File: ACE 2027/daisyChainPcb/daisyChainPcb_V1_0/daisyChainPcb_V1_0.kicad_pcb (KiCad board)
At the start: 2 copper layers, 56.5 x 97 mm, 27 parts, among them J201 Pads, J202 XT30, J203 XT30, J204 Pads, J205 Pads, J206 RJ45, J207 RJ45, U101 AP7361C-33E-13

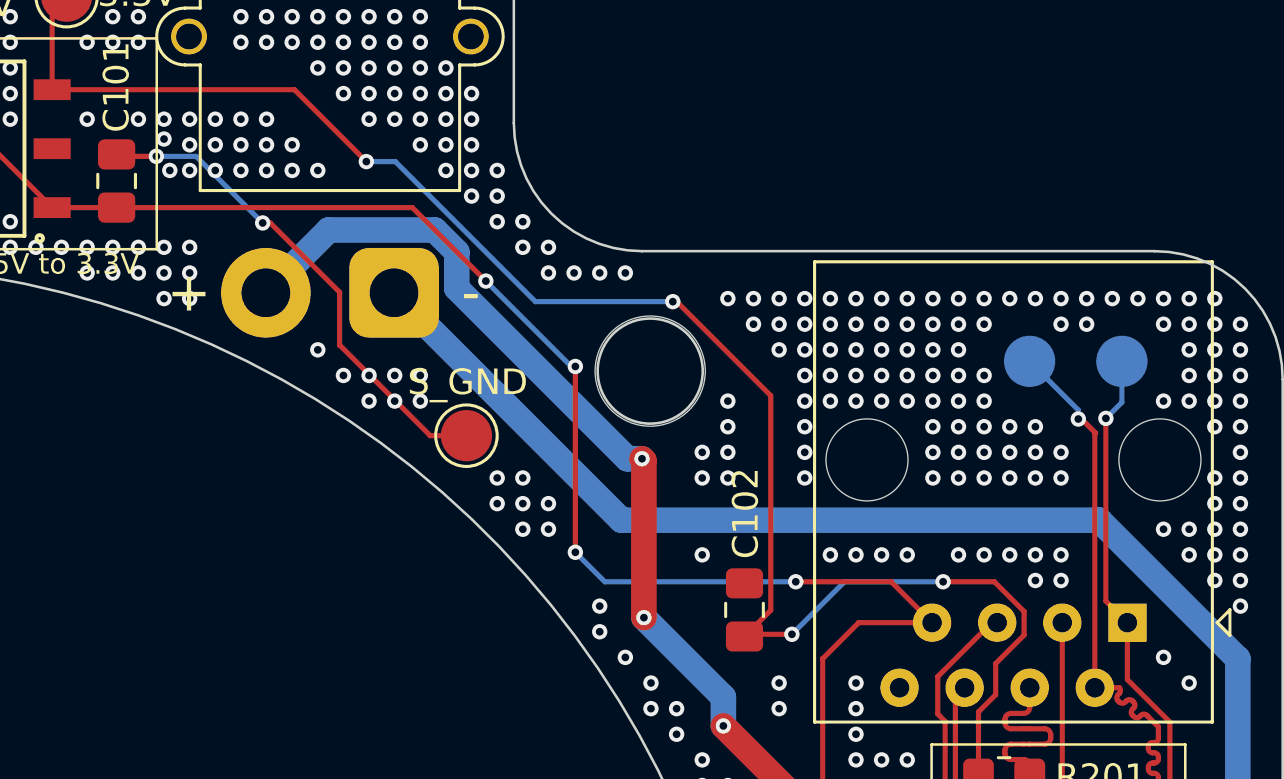
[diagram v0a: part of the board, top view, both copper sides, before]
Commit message: version finale
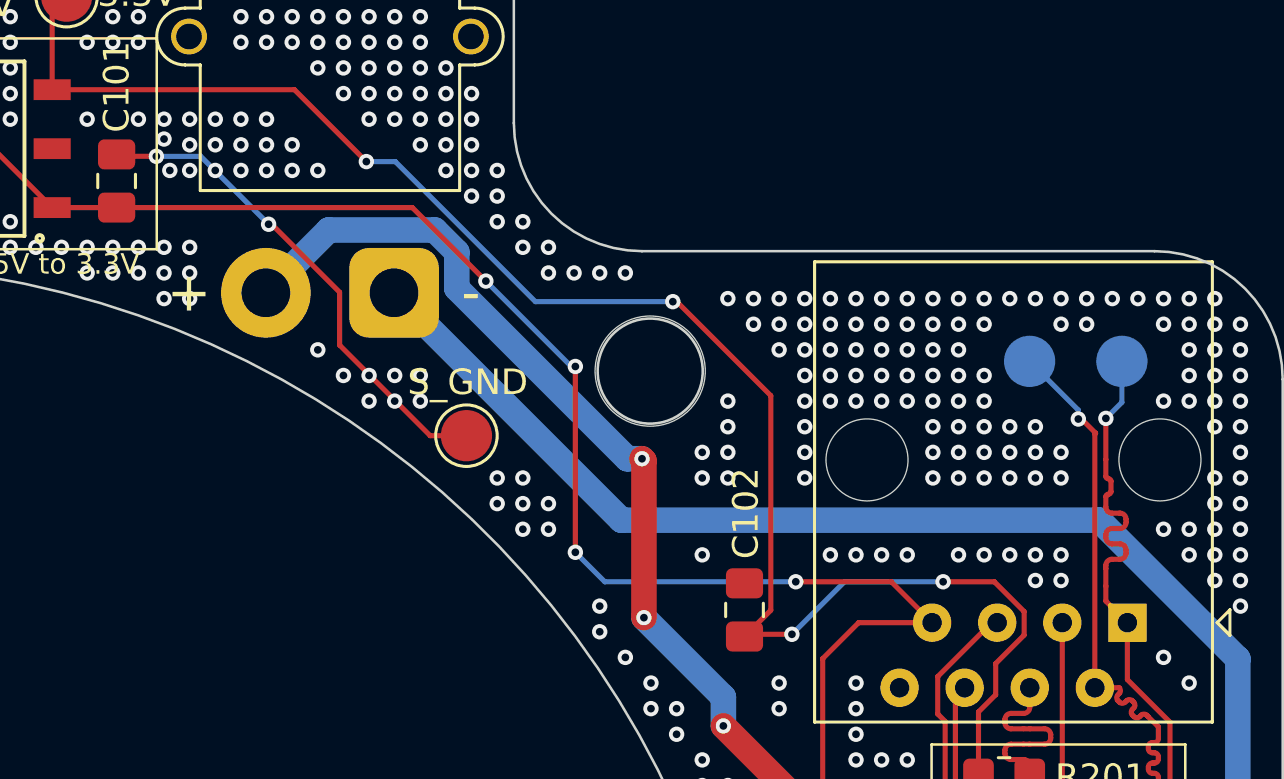
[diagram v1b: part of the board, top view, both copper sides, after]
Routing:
- net /Controle/CAN_P: track 65.3 -> 67.7 mm
